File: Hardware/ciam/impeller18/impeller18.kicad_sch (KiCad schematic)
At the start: 40 parts, among them J1 PLS-6, J2 BH1,27-10-G, J26 PLS-3, J3 PLS-3, SW1 B3F1060, SW2 MSS-12D16, SW3 MSS-12D16, U1 STM32F427ZGTx, Y1 X322516MLB4SI, Y2 KSE-7K32768KDY2400A3

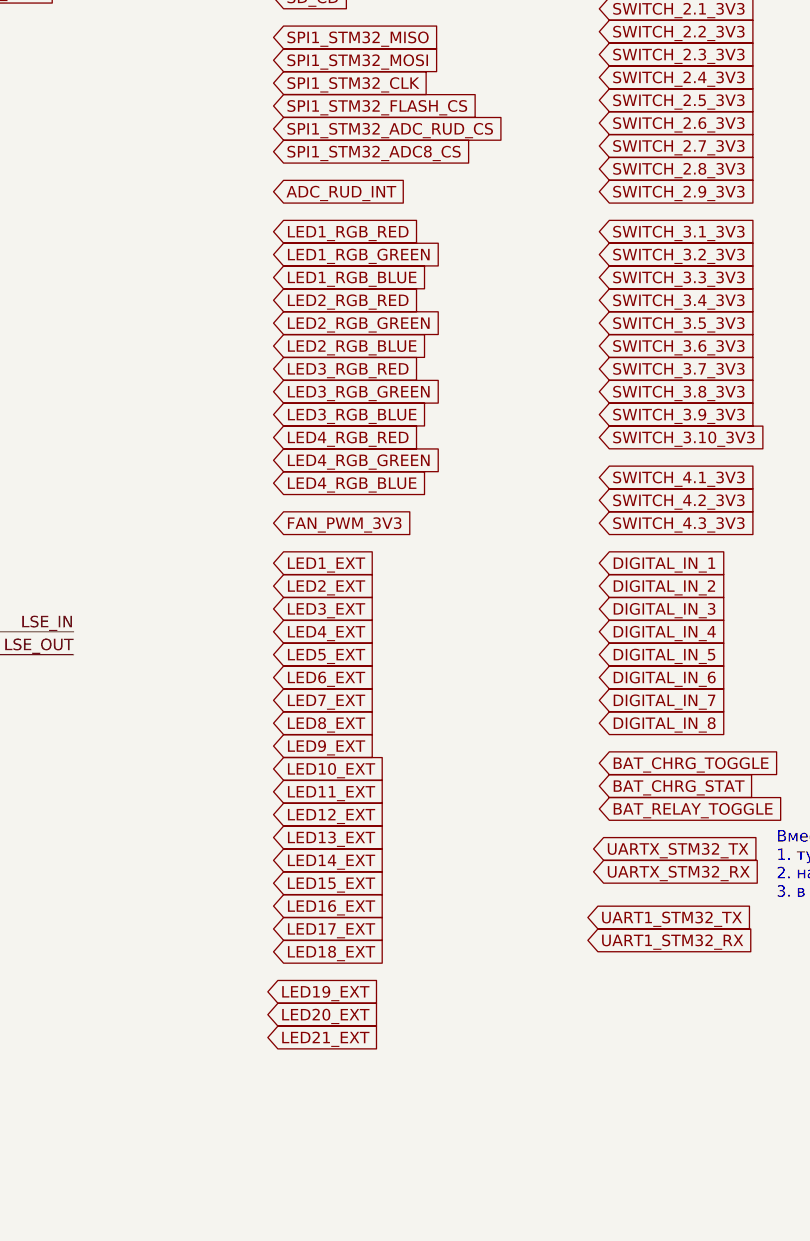
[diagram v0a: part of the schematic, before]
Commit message: added bat voltage sensor
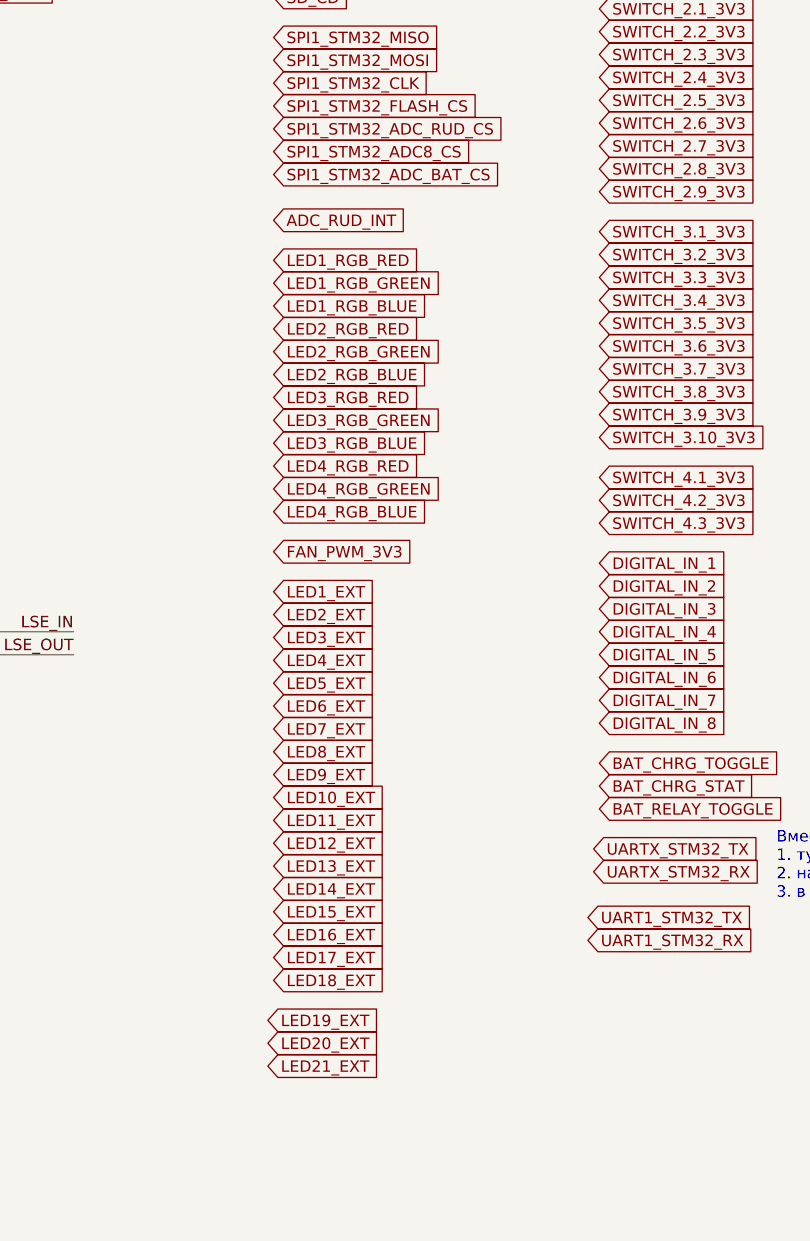
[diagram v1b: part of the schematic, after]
